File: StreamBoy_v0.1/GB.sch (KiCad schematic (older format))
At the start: 8 parts, among them J1 GB-CART, U3 LSF0204PWR, U4 LSF0204PWR, U5 LSF0204PWR, U6 LSF0204PWR, U7 LSF0204PWR, U8 LSF0204PWR, U9 LSF0204PWR

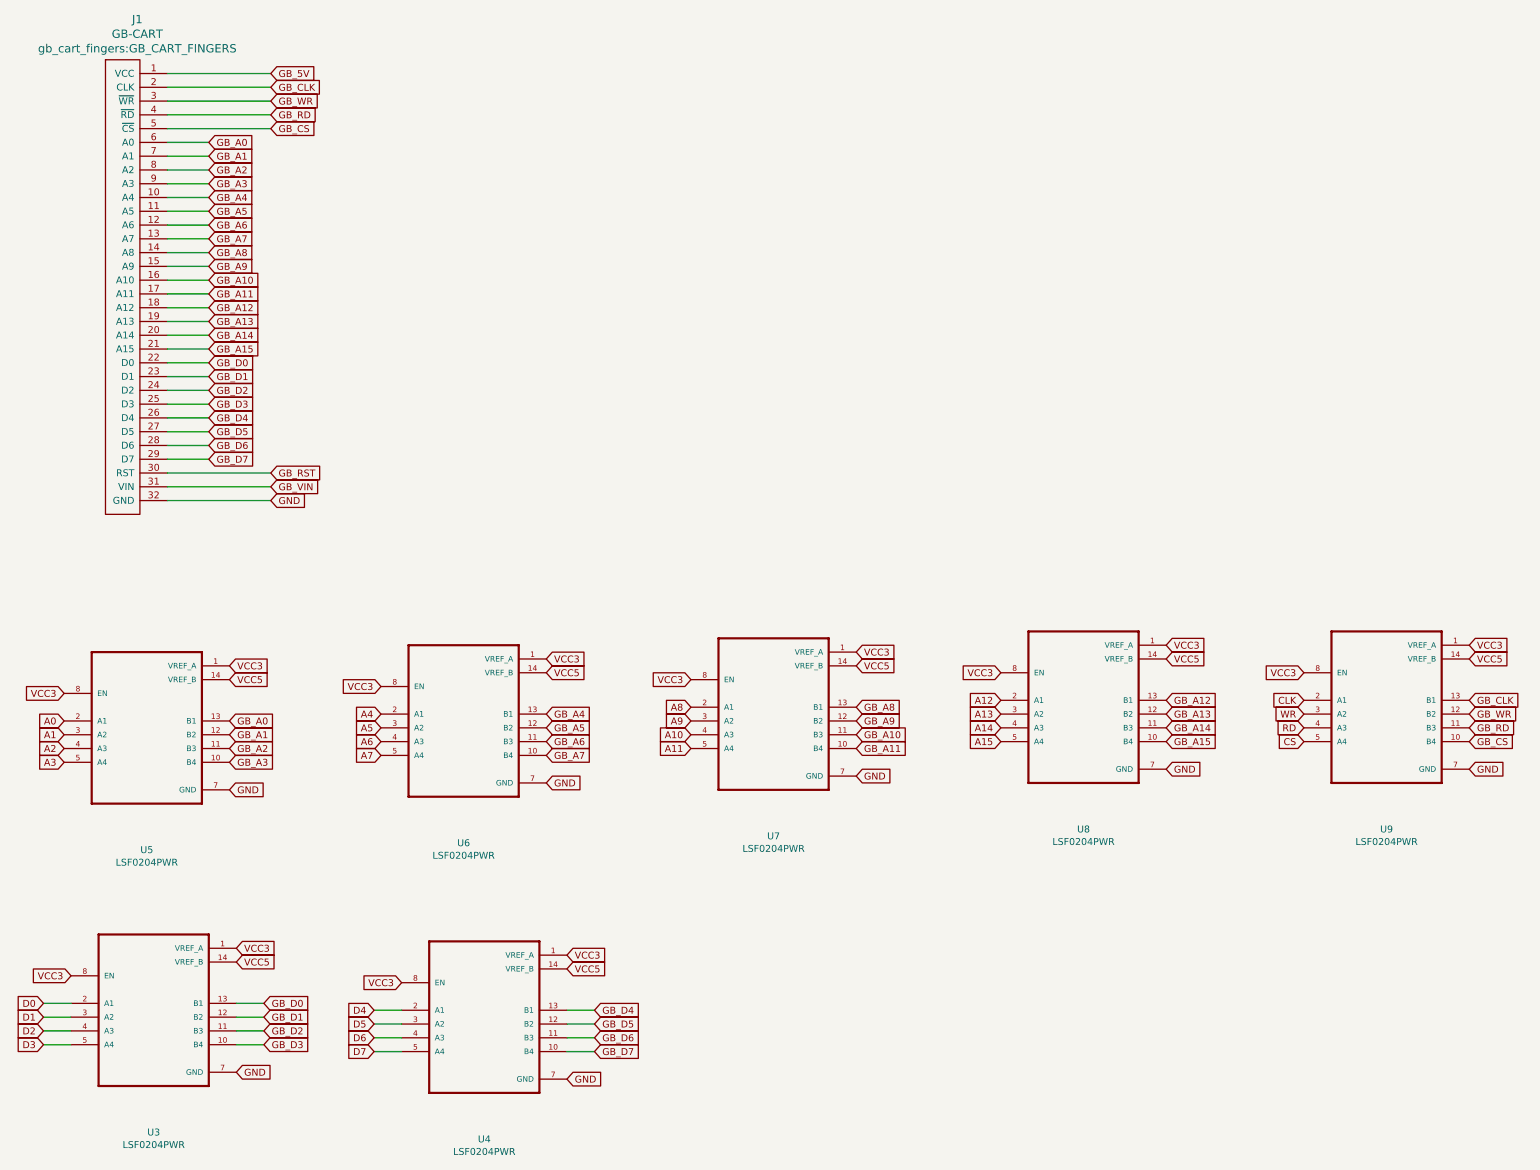
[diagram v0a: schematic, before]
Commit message: More renumbering
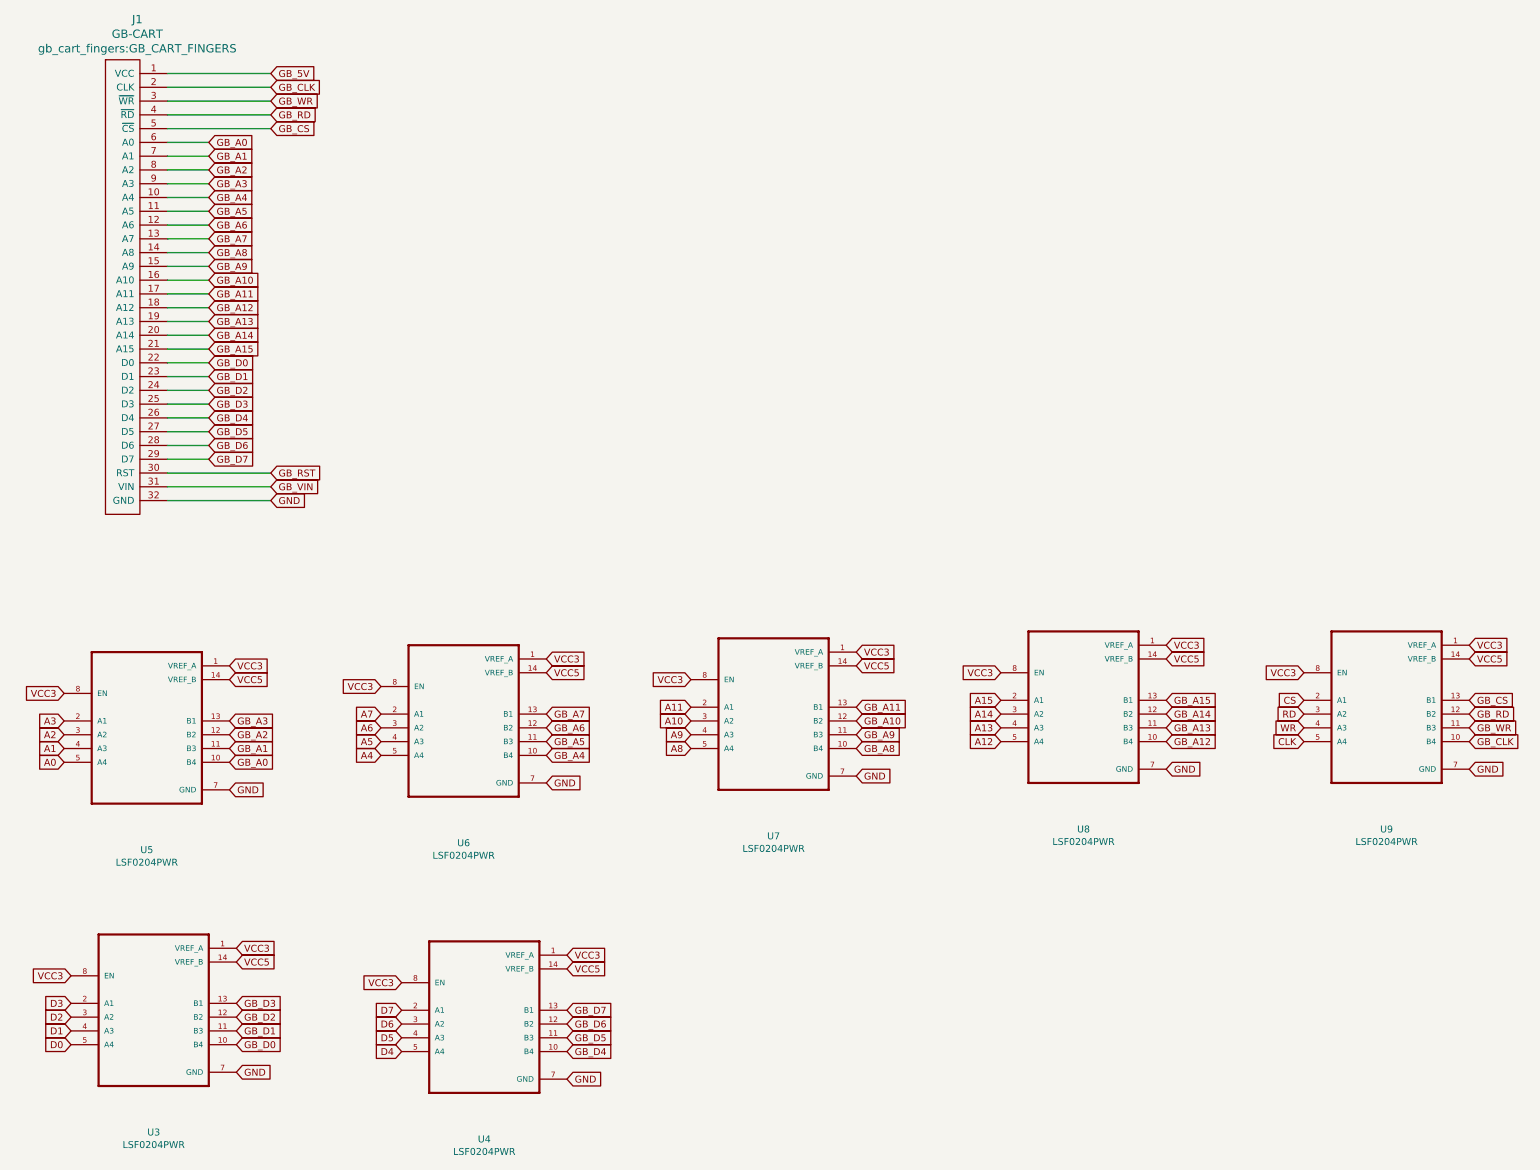
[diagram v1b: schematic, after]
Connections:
- net A0: now also U5.5 (A4); no longer U5.2 (A1)
- net A1: now also U5.4 (A3); no longer U5.3 (A2)
- net A10: now also U7.3 (A2); no longer U7.4 (A3)
- net A11: now also U7.2 (A1); no longer U7.5 (A4)
- net A12: now also U8.5 (A4); no longer U8.2 (A1)
- net A13: now also U8.4 (A3); no longer U8.3 (A2)
- net A14: now also U8.3 (A2); no longer U8.4 (A3)
- net A15: now also U8.2 (A1); no longer U8.5 (A4)
- net A2: now also U5.3 (A2); no longer U5.4 (A3)
- net A3: now also U5.2 (A1); no longer U5.5 (A4)
- net A4: now also U6.5 (A4); no longer U6.2 (A1)
- net A5: now also U6.4 (A3); no longer U6.3 (A2)
- net A6: now also U6.3 (A2); no longer U6.4 (A3)
- net A7: now also U6.2 (A1); no longer U6.5 (A4)
- net A8: now also U7.5 (A4); no longer U7.2 (A1)
- net A9: now also U7.4 (A3); no longer U7.3 (A2)
- net CLK: now also U9.5 (A4); no longer U9.2 (A1)
- net CS: now also U9.2 (A1); no longer U9.5 (A4)
- net D0: now also U3.5 (A4); no longer U3.2 (A1)
- net D1: now also U3.4 (A3); no longer U3.3 (A2)
- net D2: now also U3.3 (A2); no longer U3.4 (A3)
- net D3: now also U3.2 (A1); no longer U3.5 (A4)
- net D4: now also U4.5 (A4); no longer U4.2 (A1)
- net D5: now also U4.4 (A3); no longer U4.3 (A2)
- net D6: now also U4.3 (A2); no longer U4.4 (A3)
- net D7: now also U4.2 (A1); no longer U4.5 (A4)
- net GB_A0: now also U5.10 (B4); no longer U5.13 (B1)
- net GB_A1: now also U5.11 (B3); no longer U5.12 (B2)
- net GB_A10: now also U7.12 (B2); no longer U7.11 (B3)
- net GB_A11: now also U7.13 (B1); no longer U7.10 (B4)
- net GB_A12: now also U8.10 (B4); no longer U8.13 (B1)
- net GB_A13: now also U8.11 (B3); no longer U8.12 (B2)
- net GB_A14: now also U8.12 (B2); no longer U8.11 (B3)
- net GB_A15: now also U8.13 (B1); no longer U8.10 (B4)
- net GB_A2: now also U5.12 (B2); no longer U5.11 (B3)
- net GB_A3: now also U5.13 (B1); no longer U5.10 (B4)
- net GB_A4: now also U6.10 (B4); no longer U6.13 (B1)
- net GB_A5: now also U6.11 (B3); no longer U6.12 (B2)
- net GB_A6: now also U6.12 (B2); no longer U6.11 (B3)
- net GB_A7: now also U6.13 (B1); no longer U6.10 (B4)
- net GB_A8: now also U7.10 (B4); no longer U7.13 (B1)
- net GB_A9: now also U7.11 (B3); no longer U7.12 (B2)
- net GB_CLK: now also U9.10 (B4); no longer U9.13 (B1)
- net GB_CS: now also U9.13 (B1); no longer U9.10 (B4)
- net GB_D0: now also U3.10 (B4); no longer U3.13 (B1)
- net GB_D1: now also U3.11 (B3); no longer U3.12 (B2)
- net GB_D2: now also U3.12 (B2); no longer U3.11 (B3)
- net GB_D3: now also U3.13 (B1); no longer U3.10 (B4)
- net GB_D4: now also U4.10 (B4); no longer U4.13 (B1)
- net GB_D5: now also U4.11 (B3); no longer U4.12 (B2)
- net GB_D6: now also U4.12 (B2); no longer U4.11 (B3)
- net GB_D7: now also U4.13 (B1); no longer U4.10 (B4)
- net GB_RD: now also U9.12 (B2); no longer U9.11 (B3)
- net GB_WR: now also U9.11 (B3); no longer U9.12 (B2)
- net RD: now also U9.3 (A2); no longer U9.4 (A3)
- net WR: now also U9.4 (A3); no longer U9.3 (A2)
